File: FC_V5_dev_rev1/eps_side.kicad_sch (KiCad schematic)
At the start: 84 parts, among them IC6 LT3652IMSE#PBF, J10 INHIBIT_P2, J13 Bypass, J14 Battery Input, J15 Heater, J19 ISS_INHIBIT, J20 ISS_INHIBIT, J24 Face0, J25 Face1, J26 Face2, J27 Face4, J28 Face4, J29 INHIBIT_S2, J7 INHIBIT_P1, J8 INHIBIT_S1, Q4 FDMQ86530L, Q7 DMP2240UDM-7, Q8 DMP2240UDM-7, U10 TPS54226PWPRPWP14_2P31X2P46-L, U13 TPS7A4501DCQT, U14 INA219AxD, U15 INA219AxD, U17 LMC555CMX/NOPB, U20 74LVC1G04

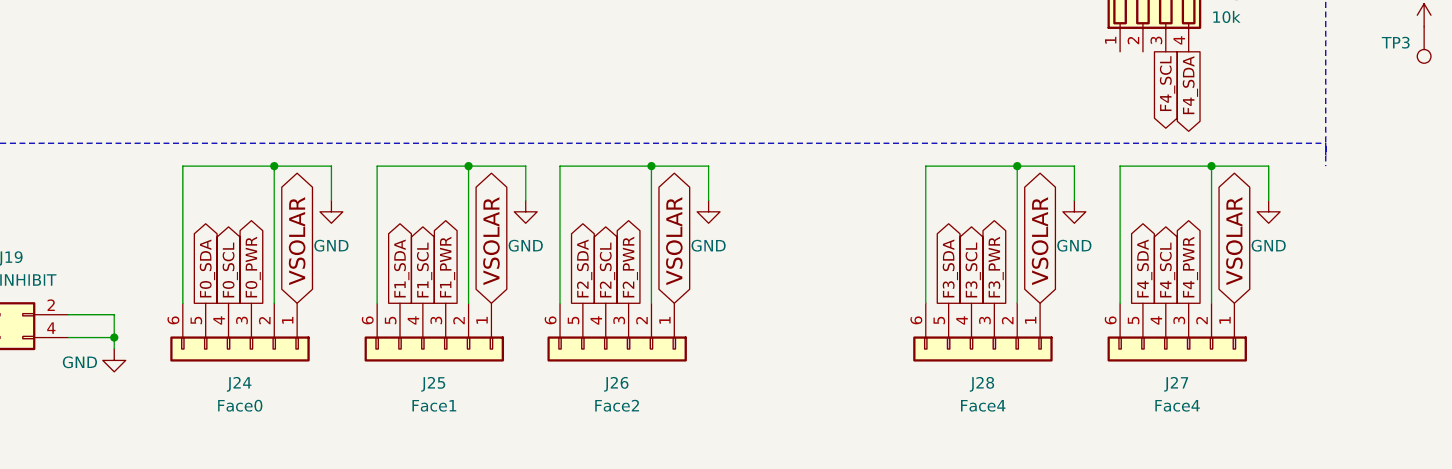
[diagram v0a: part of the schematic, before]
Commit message: Return of the Shift Register
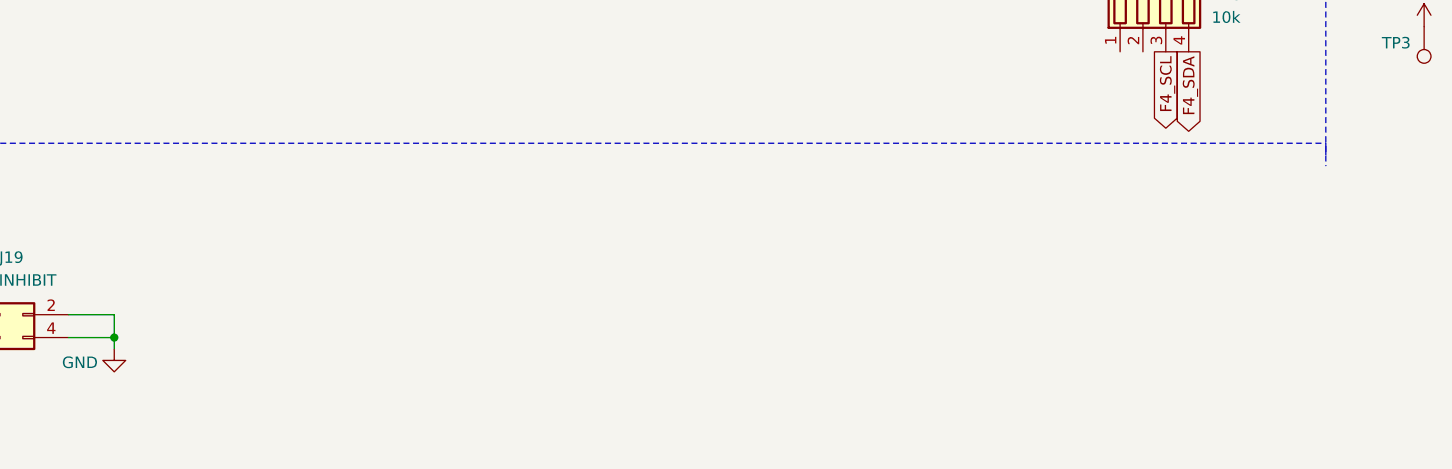
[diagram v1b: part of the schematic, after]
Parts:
- removed J24: Face0, Molex 6 pos:MOLEX_5040500691, symbol Connector_Generic:Conn_01x06
- removed J25: Face1, Molex 6 pos:MOLEX_5040500691, symbol Connector_Generic:Conn_01x06
- removed J26: Face2, Molex 6 pos:MOLEX_5040500691, symbol Connector_Generic:Conn_01x06
- removed J27, J28: Face4, Molex 6 pos:MOLEX_5040500691, symbol Connector_Generic:Conn_01x06
